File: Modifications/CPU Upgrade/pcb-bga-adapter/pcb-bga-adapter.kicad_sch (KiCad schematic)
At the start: 2 parts, among them J1 51338-1074

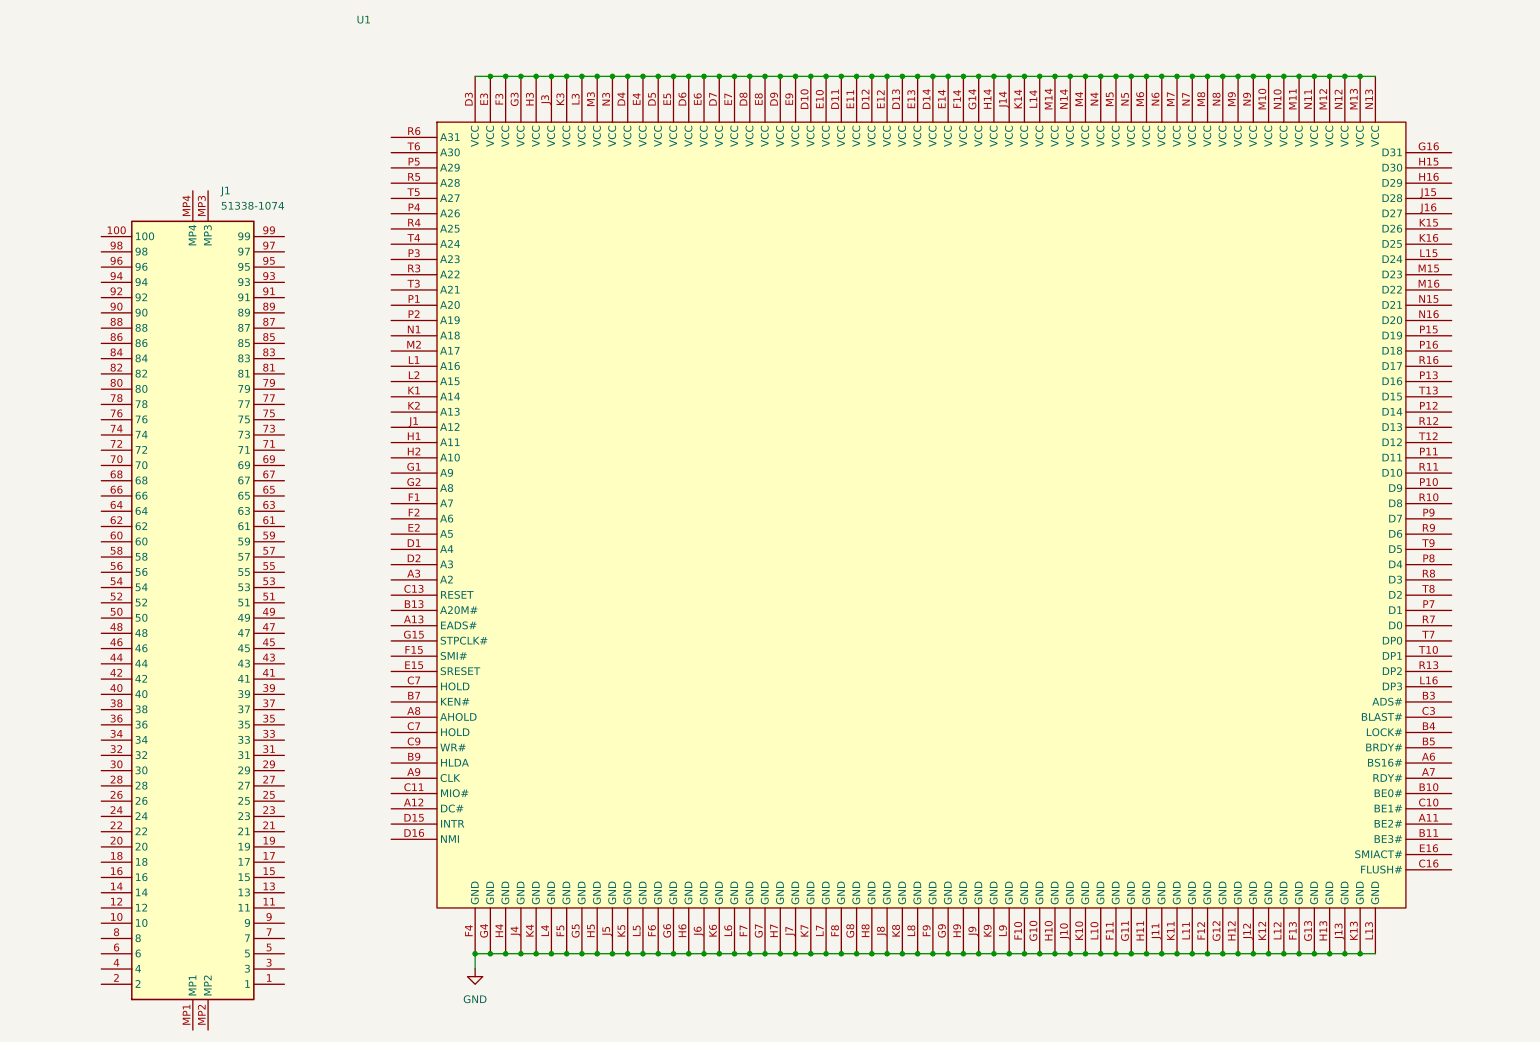
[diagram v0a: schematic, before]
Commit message: Initial commit of  cpu adapter
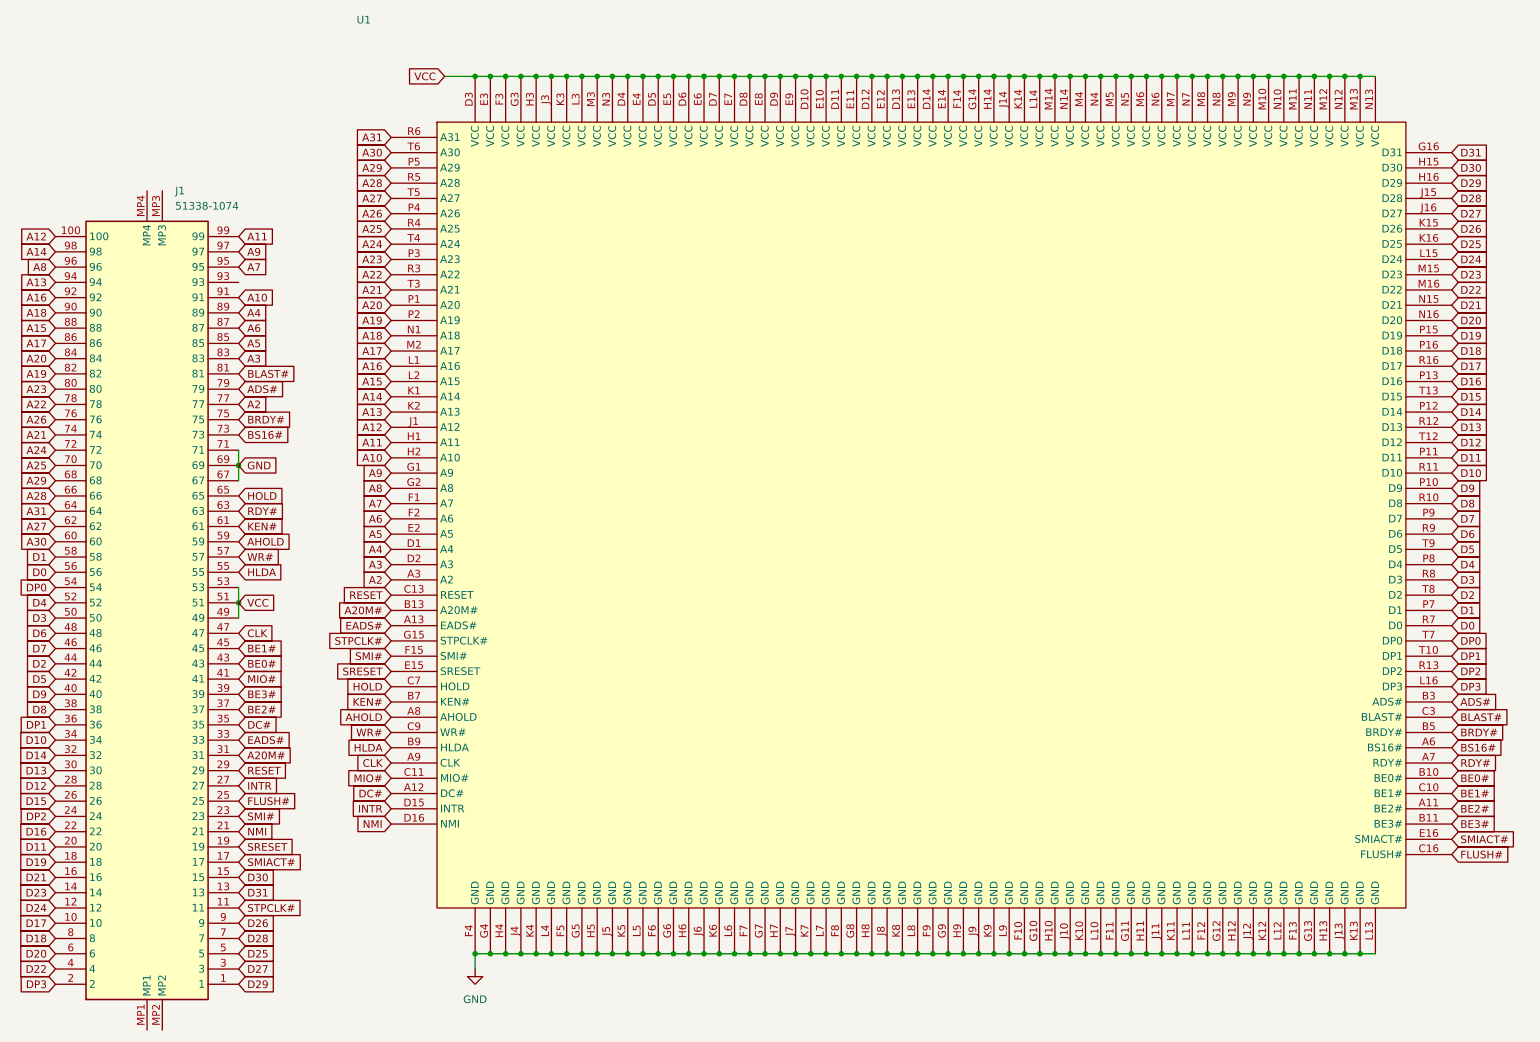
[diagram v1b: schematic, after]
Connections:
- net GND: now also J1.67, J1.69, J1.71
- net BE2#: now reaches U1.A11 (BE2#)
- net BE2#: now also J1.37
- net DC#: now reaches U1.A12 (DC#)
- net DC#: now also J1.35
- net EADS#: now reaches U1.A13 (EADS#)
- net EADS#: now also J1.33
- net A2: now reaches U1.A3 (A2)
- net A2: now also J1.77
- net BS16#: now reaches U1.A6 (BS16#)
- net BS16#: now also J1.73
- net RDY#: now reaches U1.A7 (RDY#)
- net RDY#: now also J1.63
- net AHOLD: now reaches U1.A8 (AHOLD)
- net AHOLD: now also J1.59
- net CLK: now reaches U1.A9 (CLK)
- net CLK: now also J1.47
- net BE0#: now reaches U1.B10 (BE0#)
- net BE0#: now also J1.43
- net BE3#: now reaches U1.B11 (BE3#)
- net BE3#: now also J1.39
- net A20M#: now reaches U1.B13 (A20M#)
- net A20M#: now also J1.31
- net ADS#: now reaches U1.B3 (ADS#)
- net ADS#: now also J1.79
- net BRDY#: now reaches U1.B5 (BRDY#)
- net BRDY#: now also J1.75
- net KEN#: now reaches U1.B7 (KEN#)
- net KEN#: now also J1.61
- net HLDA: now reaches U1.B9 (HLDA)
- net HLDA: now also J1.55
- net BE1#: now reaches U1.C10 (BE1#)
- net BE1#: now also J1.45
- net MIO#: now reaches U1.C11 (MIO#)
- net MIO#: now also J1.41
- net RESET: now reaches U1.C13 (RESET)
- net RESET: now also J1.29
- net FLUSH#: now reaches U1.C16 (FLUSH#)
- net FLUSH#: now also J1.25
- net BLAST#: now reaches U1.C3 (BLAST#)
- net BLAST#: now also J1.81
- net HOLD: now reaches U1.C7 (HOLD)
- net HOLD: now also J1.65
- net WR#: now reaches U1.C9 (WR#)
- net WR#: now also J1.57
- net A4: now reaches U1.D1 (A4)
- net A4: now also J1.89
- net VCC: now reaches U1.D10 (VCC), U1.D11 (VCC), U1.D12 (VCC), U1.D13 (VCC), U1.D14 (VCC), U1.D3 (VCC), U1.D4 (VCC), U1.D5 (VCC), U1.D6 (VCC), U1.D7 (VCC), U1.D8 (VCC), U1.D9 (VCC), U1.E10 (VCC), U1.E11 (VCC), U1.E12 (VCC), U1.E13 (VCC), U1.E14 (VCC), U1.E3 (VCC), U1.E4 (VCC), U1.E5 (VCC), U1.E6 (VCC), U1.E7 (VCC), U1.E8 (VCC), U1.E9 (VCC), U1.F14 (VCC), U1.F3 (VCC), U1.G14 (VCC), U1.G3 (VCC), U1.H14 (VCC), U1.H3 (VCC), U1.J14 (VCC), U1.J3 (VCC), U1.K14 (VCC), U1.K3 (VCC), U1.L14 (VCC), U1.L3 (VCC), U1.M10 (VCC), U1.M11 (VCC), U1.M12 (VCC), U1.M13 (VCC), U1.M14 (VCC), U1.M3 (VCC), U1.M4 (VCC), U1.M5 (VCC), U1.M6 (VCC), U1.M7 (VCC), U1.M8 (VCC), U1.M9 (VCC), U1.N10 (VCC), U1.N11 (VCC), U1.N12 (VCC), U1.N13 (VCC), U1.N14 (VCC), U1.N3 (VCC), U1.N4 (VCC), U1.N5 (VCC), U1.N6 (VCC), U1.N7 (VCC), U1.N8 (VCC), U1.N9 (VCC)
- net VCC: now also J1.49, J1.51, J1.53
- net INTR: now reaches U1.D15 (INTR)
- net INTR: now also J1.27
- net NMI: now reaches U1.D16 (NMI)
- net NMI: now also J1.21
- net A3: now reaches U1.D2 (A3)
- net A3: now also J1.83
- net SRESET: now reaches U1.E15 (SRESET)
- net SRESET: now also J1.19
- net SMIACT#: now reaches U1.E16 (SMIACT#)
- net SMIACT#: now also J1.17
- net A5: now reaches U1.E2 (A5)
- net A5: now also J1.85
- net A7: now reaches U1.F1 (A7)
- net A7: now also J1.95
- net SMI#: now reaches U1.F15 (SMI#)
- net SMI#: now also J1.23
- net A6: now reaches U1.F2 (A6)
- net A6: now also J1.87
- net A9: now reaches U1.G1 (A9)
- net A9: now also J1.97
- net STPCLK#: now reaches U1.G15 (STPCLK#)
- net STPCLK#: now also J1.11
- net D31: now reaches U1.G16 (D31)
- net D31: now also J1.13
- net A8: now reaches U1.G2 (A8)
- net A8: now also J1.96
- net A11: now reaches U1.H1 (A11)
- net A11: now also J1.99
- net D30: now reaches U1.H15 (D30)
- net D30: now also J1.15
- net D29: now reaches U1.H16 (D29)
- net D29: now also J1.1
- net A10: now reaches U1.H2 (A10)
- net A10: now also J1.91
- net A12: now reaches U1.J1 (A12)
- net A12: now also J1.100
- net D28: now reaches U1.J15 (D28)
- net D28: now also J1.7
- net D27: now reaches U1.J16 (D27)
- net D27: now also J1.3
- net A14: now reaches U1.K1 (A14)
- net A14: now also J1.98
- net D26: now reaches U1.K15 (D26)
- net D26: now also J1.9
- net D25: now reaches U1.K16 (D25)
- net D25: now also J1.5
- net A13: now reaches U1.K2 (A13)
- net A13: now also J1.94
- net A16: now reaches U1.L1 (A16)
- net A16: now also J1.92
- net D24: now reaches U1.L15 (D24)
- net D24: now also J1.12
- net DP3: now reaches U1.L16 (DP3)
- net DP3: now also J1.2
- net A15: now reaches U1.L2 (A15)
- net A15: now also J1.88
- net D23: now reaches U1.M15 (D23)
- net D23: now also J1.14
- net D22: now reaches U1.M16 (D22)
- net D22: now also J1.4
- net A17: now reaches U1.M2 (A17)
- net A17: now also J1.86
- net A18: now reaches U1.N1 (A18)
- net A18: now also J1.90
- net D21: now reaches U1.N15 (D21)
- net D21: now also J1.16
- net D20: now reaches U1.N16 (D20)
- net D20: now also J1.6
- net A20: now reaches U1.P1 (A20)
- net A20: now also J1.84
- net D9: now reaches U1.P10 (D9)
- net D9: now also J1.40
- net D11: now reaches U1.P11 (D11)
- net D11: now also J1.20
- net D14: now reaches U1.P12 (D14)
- net D14: now also J1.32
- net D16: now reaches U1.P13 (D16)
- net D16: now also J1.22
- net D19: now reaches U1.P15 (D19)
- net D19: now also J1.18
- net D18: now reaches U1.P16 (D18)
- net D18: now also J1.8
- net A19: now reaches U1.P2 (A19)
- net A19: now also J1.82
- net A23: now reaches U1.P3 (A23)
- net A23: now also J1.80
- net A26: now reaches U1.P4 (A26)
- net A26: now also J1.76
- net A29: now reaches U1.P5 (A29)
- net A29: now also J1.68
- net D1: now reaches U1.P7 (D1)
- net D1: now also J1.58
- net D4: now reaches U1.P8 (D4)
- net D4: now also J1.52
- net D7: now reaches U1.P9 (D7)
- net D7: now also J1.46
- net D8: now reaches U1.R10 (D8)
- net D8: now also J1.38
- net D10: now reaches U1.R11 (D10)
- net D10: now also J1.34
- net D13: now reaches U1.R12 (D13)
- net D13: now also J1.30
- net DP2: now reaches U1.R13 (DP2)
- net DP2: now also J1.24
- net D17: now reaches U1.R16 (D17)
- net D17: now also J1.10
- net A22: now reaches U1.R3 (A22)
- net A22: now also J1.78
- net A25: now reaches U1.R4 (A25)
- net A25: now also J1.70
- net A28: now reaches U1.R5 (A28)
- net A28: now also J1.66
- net A31: now reaches U1.R6 (A31)
- net A31: now also J1.64
- net D0: now reaches U1.R7 (D0)
- net D0: now also J1.56
- net D3: now reaches U1.R8 (D3)
- net D3: now also J1.50
- net D6: now reaches U1.R9 (D6)
- net D6: now also J1.48
- net DP1: now reaches U1.T10 (DP1)
- net DP1: now also J1.36
- net D12: now reaches U1.T12 (D12)
- net D12: now also J1.28
- net D15: now reaches U1.T13 (D15)
- net D15: now also J1.26
- net A21: now reaches U1.T3 (A21)
- net A21: now also J1.74
- net A24: now reaches U1.T4 (A24)
- net A24: now also J1.72
- net A27: now reaches U1.T5 (A27)
- net A27: now also J1.62
- net A30: now reaches U1.T6 (A30)
- net A30: now also J1.60
- net DP0: now reaches U1.T7 (DP0)
- net DP0: now also J1.54
- net D2: now reaches U1.T8 (D2)
- net D2: now also J1.44
- net D5: now reaches U1.T9 (D5)
- net D5: now also J1.42
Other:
- moved on the sheet: J1
